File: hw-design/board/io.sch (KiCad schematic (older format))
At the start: 33 parts, among them P4 FOOT, P5 FOOT, P6 FOOT, P7 FOOT, SW2 SP3T, U5 PCA9685

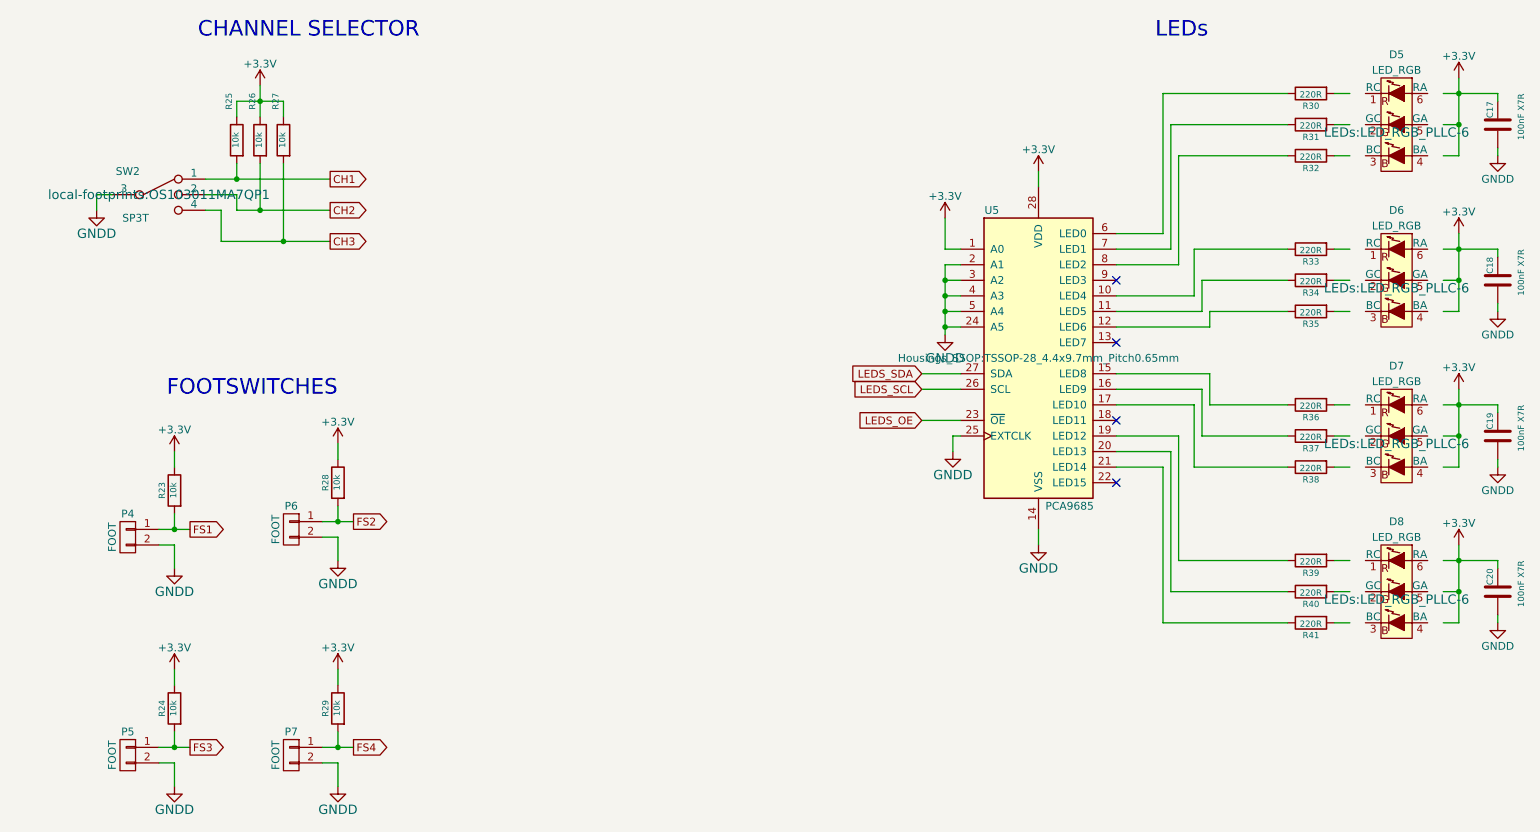
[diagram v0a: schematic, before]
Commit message: sch: kicad libray updated + missing footprints added
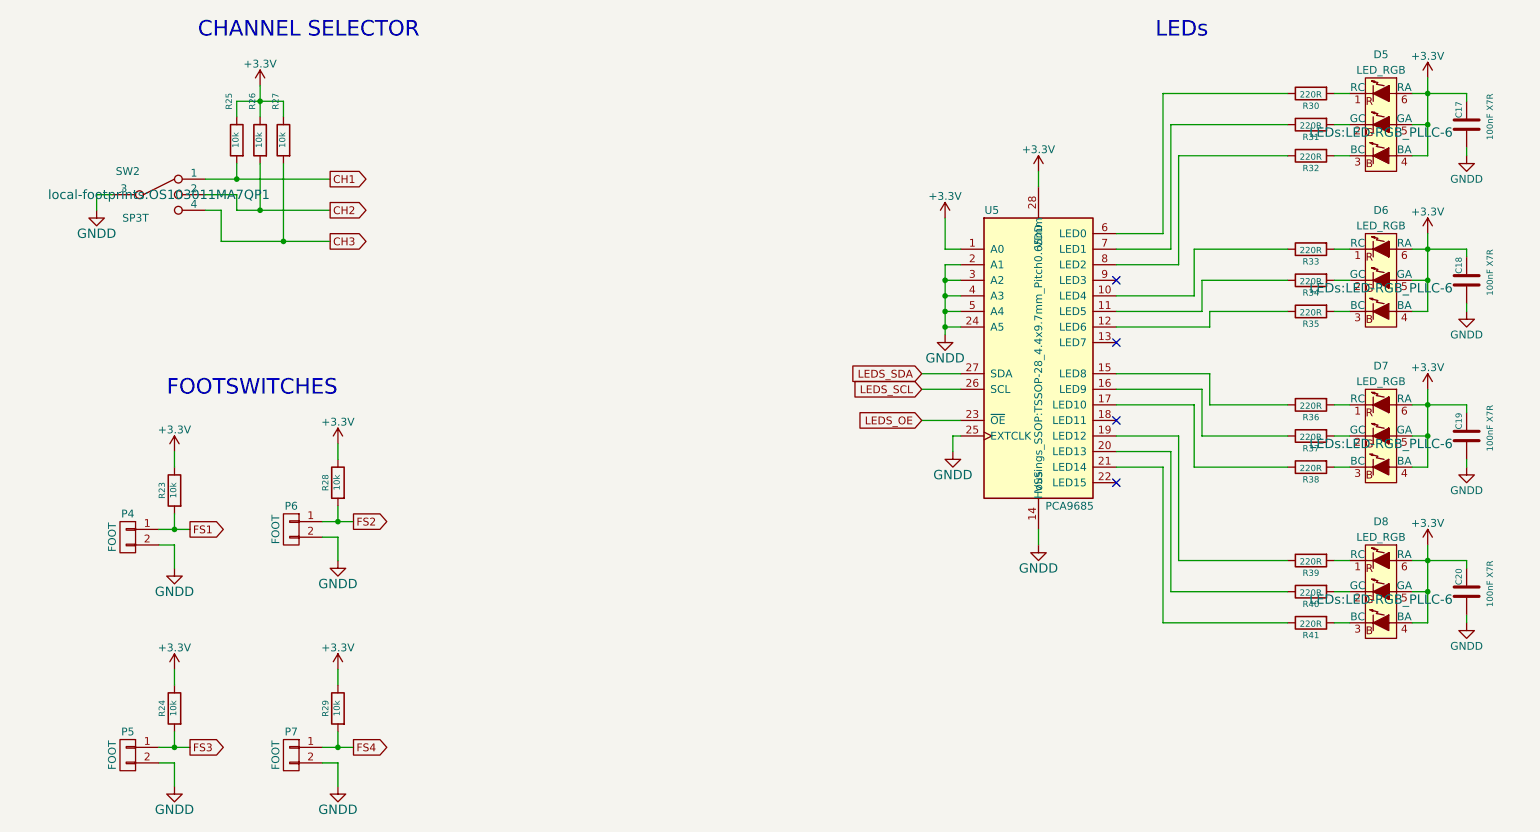
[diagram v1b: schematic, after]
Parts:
- D5, D6, D7, D8: footprint LEDs:LED_RGB_PLLC-6 -> LEDs:LED-RGB_PLLC-6
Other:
- moved on the sheet: C17, C18, C19, C20, D5, D6, D7, D8

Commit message: sch: channel selector switch is no longer used
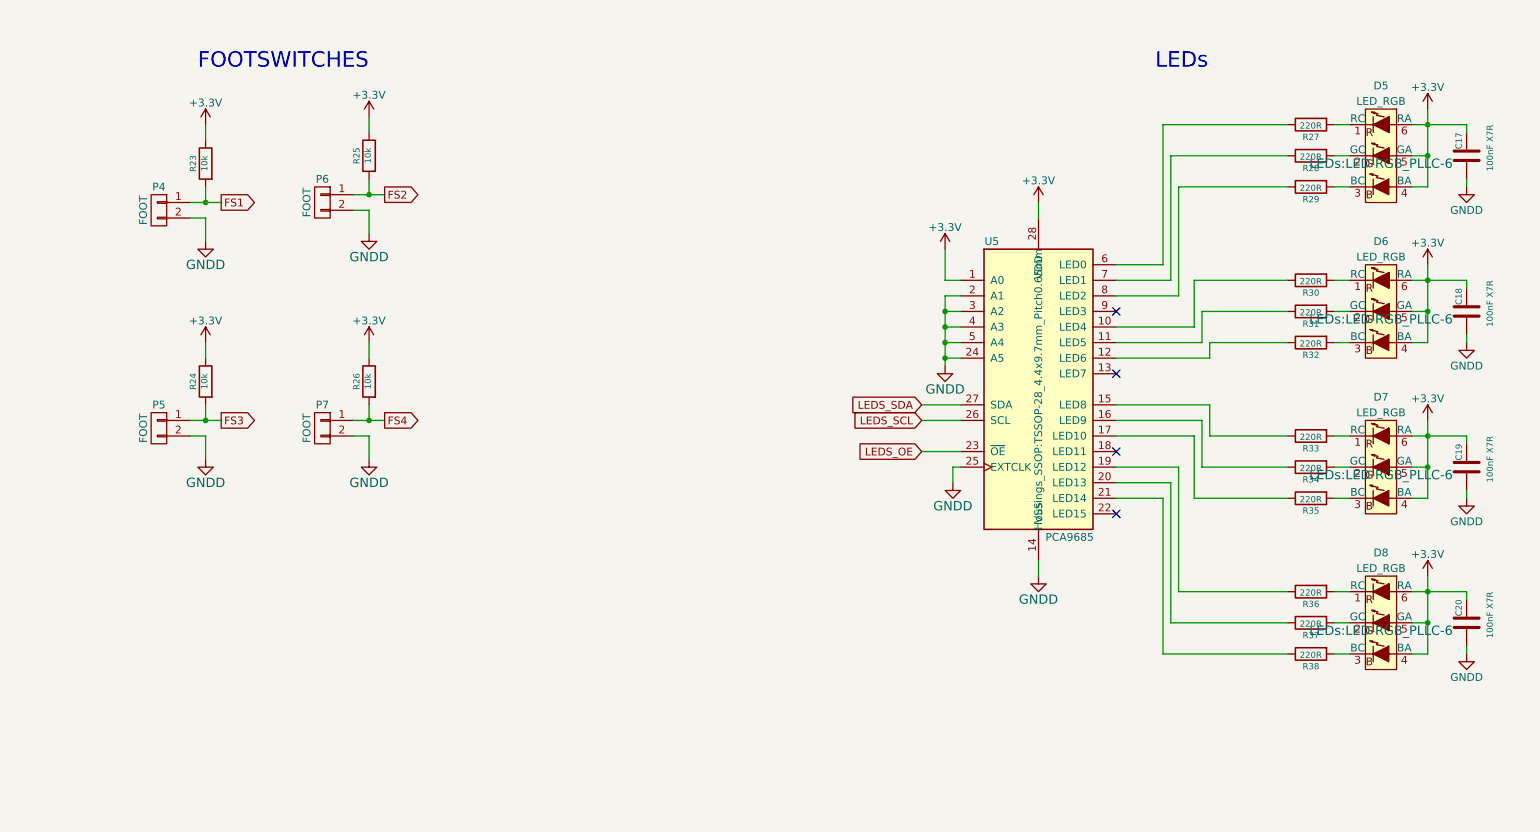
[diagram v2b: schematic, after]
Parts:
- removed R25, R26, R27: 10k, Resistors_SMD:R_0603, symbol R
- removed SW2: SP3T, local-footprints:OS103011MA7QP1, symbol SP3T
- renumbered R28 to R25, R29 to R26, R30 to R27, R31 to R28, R32 to R29, R33 to R30, R34 to R31, R35 to R32, R36 to R33, R37 to R34, R38 to R35, R39 to R36, R40 to R37, R41 to R38
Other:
- note removed: "CHANNEL SELECTOR"
- moved on the sheet: C17, C18, C19, C20, D5, D6, D7, D8, P4, P5, P6, P7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
